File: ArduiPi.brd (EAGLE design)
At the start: 85 x 56 mm, 59 parts, among them IC1 DS2482-100S, IC2 AVR-MEGA8-PPTH, J1 VIN, J3 ISP, Q1 BS170, Q2 BS170, Q3 BS170, Q4 BS170, U1 LD1117 3V3, U2 78M05, U3 TXB0108, U4 TXB0108, Y1 16MHz

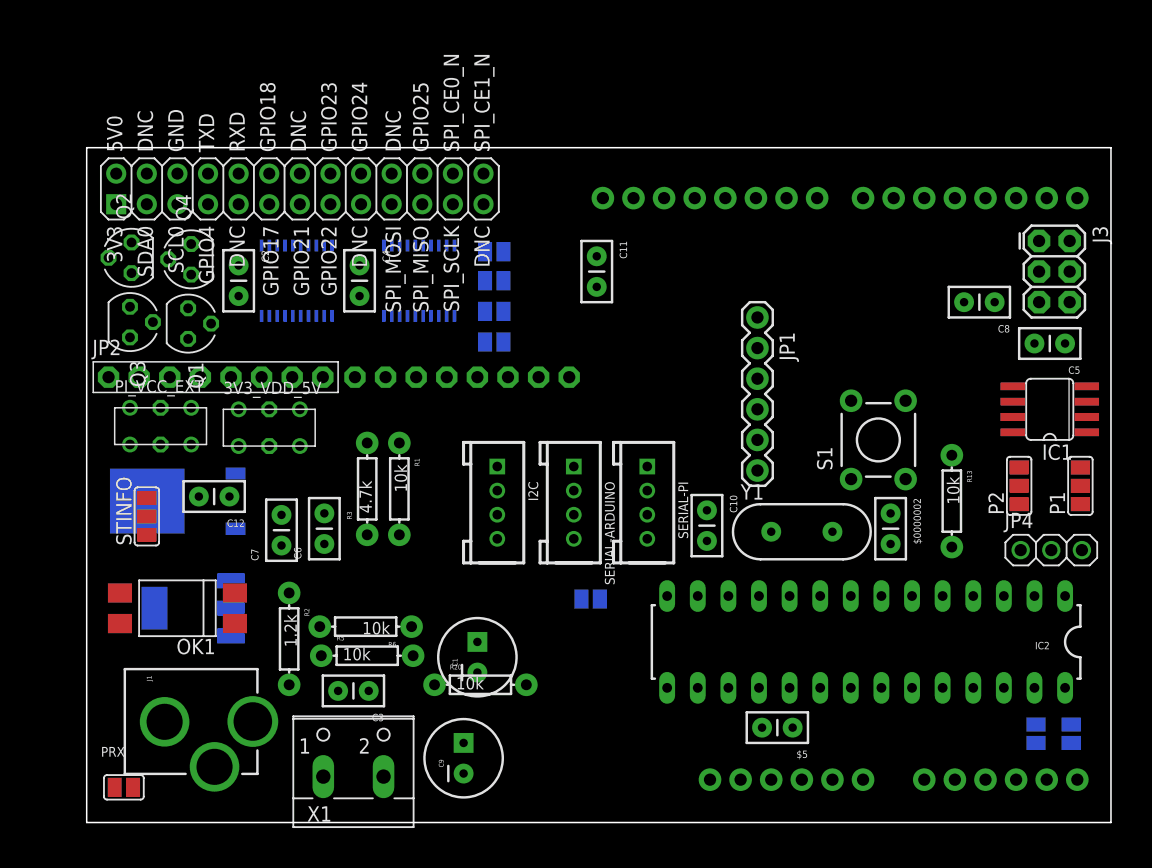
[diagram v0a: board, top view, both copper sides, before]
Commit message: Final Design
Final Design
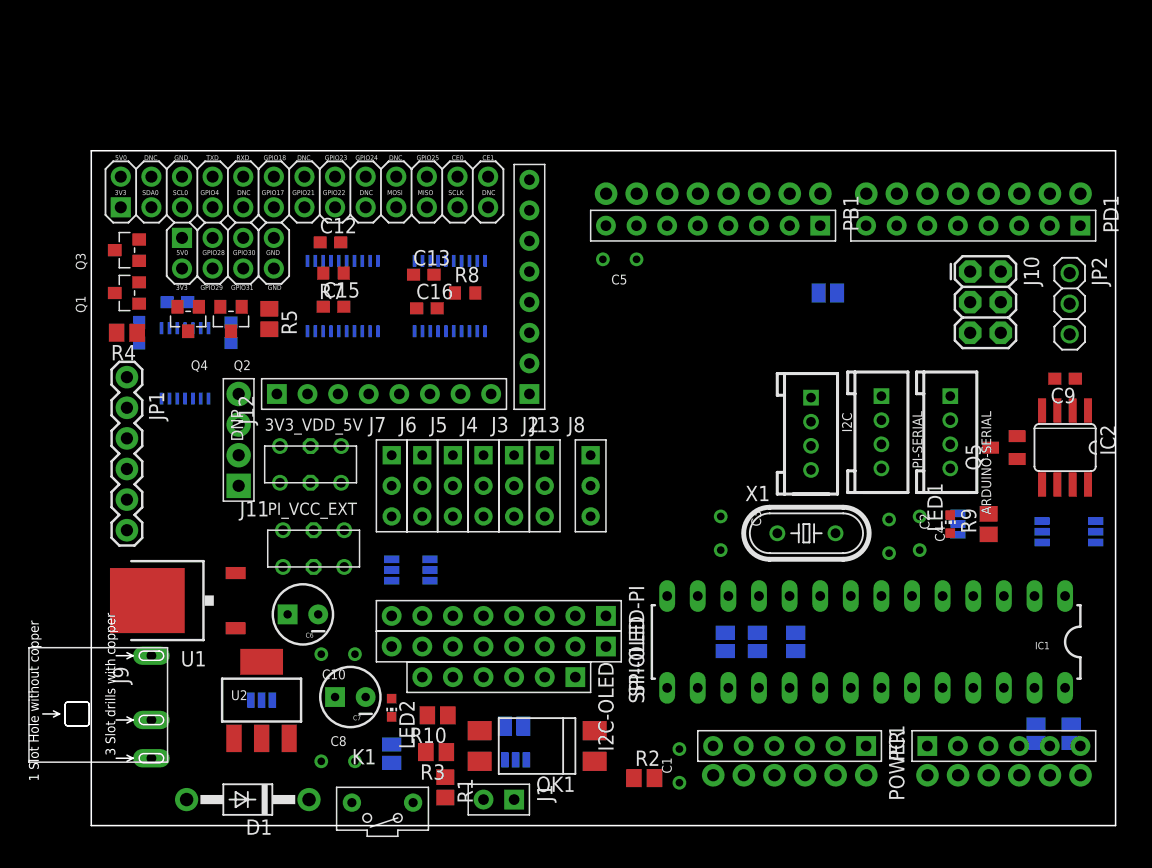
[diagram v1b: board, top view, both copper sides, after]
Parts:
- removed $0000002: 22pF, SparkFun:CAP-PTH-SMALL2
- removed $5: 0.1uF, SparkFun:CAP-PTH-SMALL2
- removed JP3: PI I/O, adafruit:1X08-BIG
- removed JP4: 1-Wire, adafruit:1X03
- removed P1, P2: (no value), Seeedstudio-Discreter.rpt:3P-SMD-2X4.8
- removed R13, R20: 10k, SparkFun:AXIAL-0.3
- removed RASPBERRY: RASPBERRYPI_BB, microbuilder:RASBERRYPI_SHIELD
- removed S1: RESET, SparkFun:TACTILE-PTH
- removed SERIAL-ARDUINO, SERIAL-PI: GROVE, Connector:4P-LEADED-2.0
- removed Y1: 16MHz, SparkFun:HC49US
- added ARDUINO-SERIAL, PI-SERIAL: GROVE, Connector:4P-LEADED-2.0
- added C13, C14, C15, C16: 0.1uF, resistor:C0603
- added D1: 1N4004, adafruit:DO41-10
- added I2C-OLED, PC1, POWER: DNP, Seeedstudio-Connector:6P-2.54
- added J10: ICSP, SparkFun:2X3
- added J11: DNP, Seeedstudio-Connector:4P-2.54-80/40MIL
- added J12, J13, PB1, PD1, SPI-OLED, SPI-OLED-PI: DNP, Seeedstudio-Connector:8P-2.54
- added J2, J4, J5, J6, J7, J8: DNP, Seeedstudio-Connector:3P-2.54
- added J9: DC-044-AH, For_Test_Albert:DC-404
- added K1: RESET, Seeedstudio-Discrete.rpt:2P-7.62X3.56-90D
- added LED1: BLUE, led:CHIP-LED0603
- added LED2: RED, led:CHIP-LED0603
- added PAD1: PAD1, Seeedstudio-Discreter.rpt:3P-SMD-2X3
- added PAD2: PAD0, Seeedstudio-Discreter.rpt:3P-SMD-2X3
- added PI-P1: PI-P1, pi:RASPBERRYPI_SHIELD
- added PLED1: PLED1, Seeedstudio-Discreter.rpt:3P-SMD-2X3
- added PLED2: PLED2, Seeedstudio-Discreter.rpt:3P-SMD-2X3
- added PSSPI: PSSPI, Seeedstudio-Discreter.rpt:3P-SMD-2X3
- added PVDD: PVDD, Seeedstudio-Discreter.rpt:2P-SMD-2X3.3
- added Q5: BSS84, transistor-small-signal:SOT23
- added R10: 180, resistor:R0805
- added R4: 4.7K, resistor:R0805
- added R7, R8: 10k, resistor:R0603
- added R9: 120, resistor:R0805
- added U5: TXB0108, adafruit:TSSOP20
- C1: value 47uF -> 0.1uF; device SparkFun:CPOL-RADIAL-100UF-25V -> Seeedstudio-Discrete.rpt:CERAMIC-1.4
- C10: value 22pF -> 0.1uF; device SparkFun:CAP-PTH-SMALL2 -> Seeedstudio-Discrete.rpt:CERAMIC-1.4
- C11, C12: device SparkFun:CAP-PTH-SMALL2 -> resistor:C0603
- C2, C3: value 0.1uF -> 22pF; device SparkFun:CAP-PTH-SMALL2 -> Seeedstudio-Discrete.rpt:CERAMIC-1.4
- C4, C5, C8: device SparkFun:CAP-PTH-SMALL2 -> Seeedstudio-Discrete.rpt:CERAMIC-1.4
- C6: value 0.1uF -> 47uF; device SparkFun:CAP-PTH-SMALL2 -> SparkFun:CPOL-RADIAL-10UF-25V
- C7: value 0.1uF -> 10uF; device SparkFun:CAP-PTH-SMALL2 -> SparkFun:CPOL-RADIAL-10UF-25V
- C9: value 10uF -> 0.1uF; device SparkFun:CPOL-RADIAL-100UF-25V -> resistor:C0603
- IC1: value DS2482-100S -> AVR-MEGA8-PPTH; device 1wire:SO08 -> SparkFun:DIL28-3
- IC2: value AVR-MEGA8-PPTH -> DS2482-100S; device SparkFun:DIL28-3 -> 1wire:SO08
- J1: value VIN -> Teleinfo; device SparkFun:POWER_JACK_PTH_LOCK -> Seeedstudio-Connector:2P-2.54
- J3: value ISP -> DNP; device SparkFun:2X3 -> Seeedstudio-Connector:3P-2.54
- JP2: value PI I/O -> 1-Wire; device adafruit:1X08-BIG -> adafruit:1X03
- PCLK: value (none) -> PCLK
- PMISO: value (none) -> PMISO
- PMOSI: value (none) -> PMOSI
- PRX: value (none) -> PRX
- PSCL: value (none) -> PSCL
- PSDA: value (none) -> PSDA
- PSS: value (none) -> PSS; device Seeedstudio-Discreter.rpt:2P-SMD-2X3.3 -> Seeedstudio-Discreter.rpt:3P-SMD-2X3
- PTX: value (none) -> PTX
- Q1, Q2, Q3, Q4: value BS170 -> BSS138; device transistor-small-signal:SOT54E -> Seeedstudio-Discreter.rpt:SOT23
- R1: value 10k -> 1.2k; device SparkFun:AXIAL-0.3 -> resistor:R0805
- R2: value 1.2k -> 10k; device SparkFun:AXIAL-0.3 -> resistor:R0805
- R3: device SparkFun:AXIAL-0.3 -> resistor:R0805
- R5: value 10k -> 4.7K; device SparkFun:AXIAL-0.3 -> resistor:R0805
- R6: device SparkFun:AXIAL-0.3 -> resistor:R0603
- STINFO: value (none) -> STINFO; device Seeedstudio-Discreter.rpt:3P-SMD-2X4.8 -> Seeedstudio-Discreter.rpt:3P-SMD-2X3
- U1: value LD1117 3V3 -> 78M05; device Seeedstudio-IC:SOT-223 -> SeedStudio-IC:TO252
- U2: value 78M05 -> LD1117 3V3; device SeedStudio-IC:TO252 -> Seeedstudio-IC:SOT-223
- U3: value TXB0108 -> TXB0104; device adafruit:TSSOP20 -> adafruit:TSSOP14
- X1: value (none) -> 16Mhz; device _c2h:W237-102 -> Seeedstudio-Discrete.rpt:HC49/S
- moved JP2 71.1 mm to (81.7, 43.1), turned to 270 degrees
- moved C8 66.5 mm to (21.0, 5.08), turned to 0 degrees
- moved C9 59.0 mm to (81.3, 36.8), turned to 180 degrees
- moved C2 58.5 mm to (66.7, 23.7)
- moved JP1 52.6 mm to (3.43, 37.0)
- moved C4 51.5 mm to (69.2, 24.0)
- moved J3 48.1 mm to (35.6, 27.9), turned to 0 degrees
- moved X1 42.1 mm to (59.8, 24.0)
- moved PMOSI 37.6 mm to (53.1, 15.0), turned to 270 degrees
- moved C5 37.6 mm to (44.3, 46.7)
- moved PCLK 37.1 mm to (58.9, 15.0), turned to 270 degrees
- moved PMISO 37.1 mm to (55.8, 15.0), turned to 270 degrees
- moved STINFO 36.7 mm to (35.7, 5.21), flipped to the bottom, turned to 0 degrees
- moved C11 35.0 mm to (7.62, 43.2), flipped to the bottom, turned to 180 degrees
- moved J1 34.9 mm to (34.3, 1.91)
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- renumbered SCL to PSCL, SDA to PSDA
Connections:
- new net GPIO28: PI-P1.P5.3, U3.2
- new net GPIO29: PI-P1.P5.4, U3.3
- new net GPIO30: PI-P1.P5.5, U3.4
- new net GPIO31: PI-P1.P5.6, U3.5
- new net IO28: J11.1, U3.13
- new net IO29: J11.2, U3.12
- new net IO30: J11.3, U3.11
- new net IO31: J11.4, U3.10
- new net N$14: J1.2, R1.2
- new net N$15: IC2.6, Q5.1
- new net N$16: PLED1.2, R9.1
- new net N$17: LED1.A, R9.2
- new net N$18: LED2.A, R10.2
- new net N$19: R6.1, U3.8
- new net N$20: PLED2.2, R10.1
- new net SSPI: PSSPI.2, SPI-OLED-PI.8
- net 3V3: now also POWER.5
- net 3V3-EXT: now also C10.2, U2.2, U2.TER; no longer C7.1, U1.TER
- net 3V3-PI: now also C11.1, C12.1, C13.1, PI-P1.1, PI-P1.P5.2, Q3.1, Q4.1, R6.2, R7.2, R8.2, U3.1, U5.2; no longer C2.1, C3.1, Q2.G, Q4.G, R5.P$2, R6.P$2, RASPBERRY.1, U3.2
- net 5V-EXT: now also C7.1, C8.2, PLED2.1, PVDD.2, U1.2, U2.3; no longer C12.1, C9.1, U1.3, U2.2
- net 5V-PI: now also PI-P1.2, PI-P1.P5.1, PLED2.3; no longer RASPBERRY.2
- net AD0: now also IC1.23, PC1.1; no longer IC2.23
- net AD1: now also IC1.24, PC1.2; no longer IC2.24
- net AD2: now also IC1.25, PC1.3; no longer IC2.25
- net AD3: now also IC1.26, PC1.4; no longer IC2.26
- net AD4/SDA: now also IC1.27, PC1.5; no longer IC2.27
- net AD5/SCL: now also IC1.28, PC1.6; no longer IC2.28
- net AREF: now also C5.2, PB1.8; no longer C11.1
- net CE0: now also J13.6, PSS.3, PSSPI.3, U5.14; no longer JP3.6, PSS.1, U4.14
- net CE1: now also J13.7, PSS.1, PSSPI.1, U5.13; no longer JP3.7, U4.13
- net CE3: now also J13.8, U5.12; no longer JP3.8, U4.12
- net D0/RX-I: now also ARDUINO-SERIAL.1, IC1.2, PD1.1; no longer IC2.2
- net D1/TX-O: now also ARDUINO-SERIAL.2, IC1.3, PD1.2; no longer IC2.3
- net D10/SS: now also IC1.16, J6.3, PB1.3, SPI-OLED.8; no longer IC2.16
- net D11/MOSI: now also IC1.17, J10.4, J7.3, PB1.4, SPI-OLED.4; no longer IC2.17, J3.4
- net D12/MISO: now also IC1.18, J10.1, PB1.5; no longer IC2.18, J3.1
- net D13/SCK: now also IC1.19, J10.3, PB1.6, PLED1.1, SPI-OLED.5; no longer IC2.19, J3.3
- net D2: now also IC1.4, PD1.3, PLED1.3; no longer IC2.4
- net D3: now also IC1.5, J2.3, PD1.4; no longer IC2.5
- net D4: now also I2C-OLED.4, IC1.6, PD1.5; no longer IC2.6
- net D5: now also IC1.11, J3.3, PD1.6; no longer IC2.11
- net D6: now also IC1.12, J4.3, PD1.7; no longer IC2.12
- net D7: now also IC1.13, PD1.8, SPI-OLED.7; no longer IC2.13
- net D8: now also IC1.14, PB1.1, SPI-OLED.6; no longer IC2.14
- net D9: now also IC1.15, J5.3, PB1.2; no longer IC2.15
- net DTR: now also C1.2; no longer C8.1
- net GND: now also ARDUINO-SERIAL.4, C13.2, C14.2, C15.2, C16.2, C6.2, C8.1, I2C-OLED.3, IC1.22, IC1.8, IC2.3, J10.6, J2.2, J3.2, J4.2, J5.2, J6.2, J7.2, J8.2, J9.-, J9.CDN, JP2.3, K1.P$1, LED1.C, LED2.C, PAD1.1, PAD2.1, PB1.7, PI-P1.6, PI-P1.P5.7, PI-P1.P5.8, PI-SERIAL.4, POWER.2, POWER.3, SPI-OLED-PI.1, SPI-OLED.1, U1.3, U2.1, U3.7, U5.11; no longer $0000002.1, $5.1, C1.2, C6.1, IC1.3, IC2.22, IC2.8, J1.GND, J1.GNDBREAK, J3.6, P1.1, P2.1, RASPBERRY.6, S1.1, S1.2, SERIAL-ARDUINO.4, SERIAL-PI.4, U1.1, U2.3, U3.11
- net GPIO17: now also PI-P1.11, U4.3; no longer RASPBERRY.11, U3.3
- net GPIO18: now also PI-P1.12, U4.4; no longer RASPBERRY.12, U3.4
- net GPIO21: now also PI-P1.13, U4.5; no longer RASPBERRY.13, U3.5
- net GPIO22: now also PI-P1.15, U4.6; no longer RASPBERRY.15, U3.6
- net GPIO23: now also PI-P1.16, U4.7; no longer RASPBERRY.16, U3.7
- net GPIO24: now also PI-P1.18, U4.8; no longer RASPBERRY.18, U3.8
- net GPIO25: now also PI-P1.22, U4.9; no longer RASPBERRY.22, U3.9
- net GPIO4: now also PI-P1.7, U4.1; no longer RASPBERRY.7, U3.1
- net IO17: now also J12.2, U4.18; no longer JP2.2, U3.18
- net IO18: now also J12.3, J8.3, U4.17; no longer JP2.3, U3.17
- net IO21: now also J12.4, U4.16; no longer JP2.4, U3.16
- net IO22: now also J12.5, U4.15; no longer JP2.5, U3.15
- net IO23: now also J12.6, U4.14; no longer JP2.6, U3.14
- net IO24: now also J12.7, SPI-OLED-PI.6, U4.13; no longer JP2.7, U3.13
- net IO25: now also J12.8, SPI-OLED-PI.7, U4.12; no longer JP2.8, U3.12
- net IO4: now also J12.1, U4.20; no longer JP2.1, U3.20
- net MISO: now also J13.4, U5.16; no longer JP3.4, U4.16
- net MISO-PI: now also PI-P1.21, U5.5; no longer RASPBERRY.21
- net MOSI: now also J13.3, SPI-OLED-PI.4, U5.17; no longer JP3.3, U4.17
- net MOSI-PI: now also PI-P1.19, U5.4; no longer RASPBERRY.19
- net N$1: now also R3.1; no longer R3.P$1
- net N$10: now also JP1.VCC, PVDD.1; no longer R2.P$2, X1.1
- net N$11: now also IC2.7, PAD1.2; no longer IC1.7, P1.2
- net N$12: now also D1.A, J9.+; no longer U1.2
- net N$13: now also R8.1, U5.10; no longer R6.P$1, U4.10
- net N$2: now also IC2.8, PAD2.2; no longer IC1.8, P2.2
- net N$3: now also C3.1, IC1.10, X1.1; no longer $0000002.2, IC2.9, Y1.2
- net N$4: now also C2.1, IC1.9, X1.2; no longer C10.2, IC2.10, Y1.1
- net N$5: now also Q1.3, Q3.3; no longer Q2.D, Q3.D
- net N$6: now also Q2.3, Q4.3; no longer Q1.D, Q4.D
- net N$7: now also R7.1, U4.10; no longer R5.P$1, U3.10
- net N$8: now also R1.1; no longer R2.P$1
- net N$9: now also J1.1; no longer X1.2
- net OW: now also IC2.2, JP2.2, Q5.3; no longer IC1.2, JP4.2
- net RESET: now also C1.1, IC1.1, J10.5, K1.P$2, POWER.6, R2.2; no longer C8.2, IC2.1, J3.5, R13.P$1, S1.3, S1.4
- net RXD: now also J13.2, PI-SERIAL.1, U5.18; no longer JP3.2, U4.18
- net RXD-PI: now also PI-P1.10, U5.3; no longer RASPBERRY.10
- net SCL: now also I2C-OLED.5, IC2.4, Q2.2, R5.1; no longer IC1.4, Q1.S, R20.P$2
- net SCL-PI: now also PI-P1.5, Q4.2; no longer Q4.S, RASPBERRY.5
- net SCLK: now also J13.5, SPI-OLED-PI.5, U5.15; no longer JP3.5, U4.15
- net SCLK-PI: now also PI-P1.23, U5.6; no longer RASPBERRY.23
- net SDA: now also I2C-OLED.6, IC2.5, Q1.2, R4.1; no longer IC1.5, Q3.S, R1.P$1
- net SDA-PI: now also PI-P1.3, Q3.2; no longer Q2.S, RASPBERRY.3
- net SPI_CE0: now also PI-P1.24, U5.7; no longer RASPBERRY.24
- net SPI_CE1: now also PI-P1.26, U5.8; no longer RASPBERRY.26
- net TXD: now also J13.1, PI-SERIAL.2, U5.20; no longer JP3.1, U4.20
- net TXD-PI: now also PI-P1.8, U5.1; no longer RASPBERRY.8
- net VDD: now also ARDUINO-SERIAL.3, C14.1, C15.1, C16.1, C9.1, I2C-OLED.1, IC1.20, IC1.7, IC2.1, J10.2, J2.1, J3.1, J4.1, J5.1, J6.1, J7.1, J8.1, JP2.1, PAD1.3, PAD2.3, PI-SERIAL.3, POWER.4, Q1.1, Q2.1, Q5.2, R2.1, R3.2, R4.2, R5.2, SPI-OLED-PI.3, SPI-OLED.3, U3.14, U5.19; no longer $5.2, C5.2, C6.2, IC1.1, IC2.20, IC2.7, J3.2, JP4.1, P1.3, P2.3, Q1.G, Q3.G, R1.P$2, R13.P$2, R20.P$1, R3.P$2, SERIAL-ARDUINO.3, SERIAL-PI.3, U3.19
- net VIN: now also C6.1, D1.C, POWER.1, U1.1; no longer C1.1, J1.PWR, U2.1
